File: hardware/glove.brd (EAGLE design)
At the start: 50.8 x 36.8 mm, 91 parts, among them J1 TC2030-JLINK-NL, J2 MICRO_USB_B_JST_MC5BR3-M404-4S, P1 DMP1045U, T0 WIREPAD1,6/0,8, T1 WIREPAD1,6/0,8, T2 WIREPAD1,6/0,8, T3 WIREPAD1,6/0,8, U1 NRF51822QF, U2 BNO055, U3 AT42QT1070, U4 MCP73831, U5 LP3855EMP-ADJ, X1 ABS05-32.768KHZ-9-T

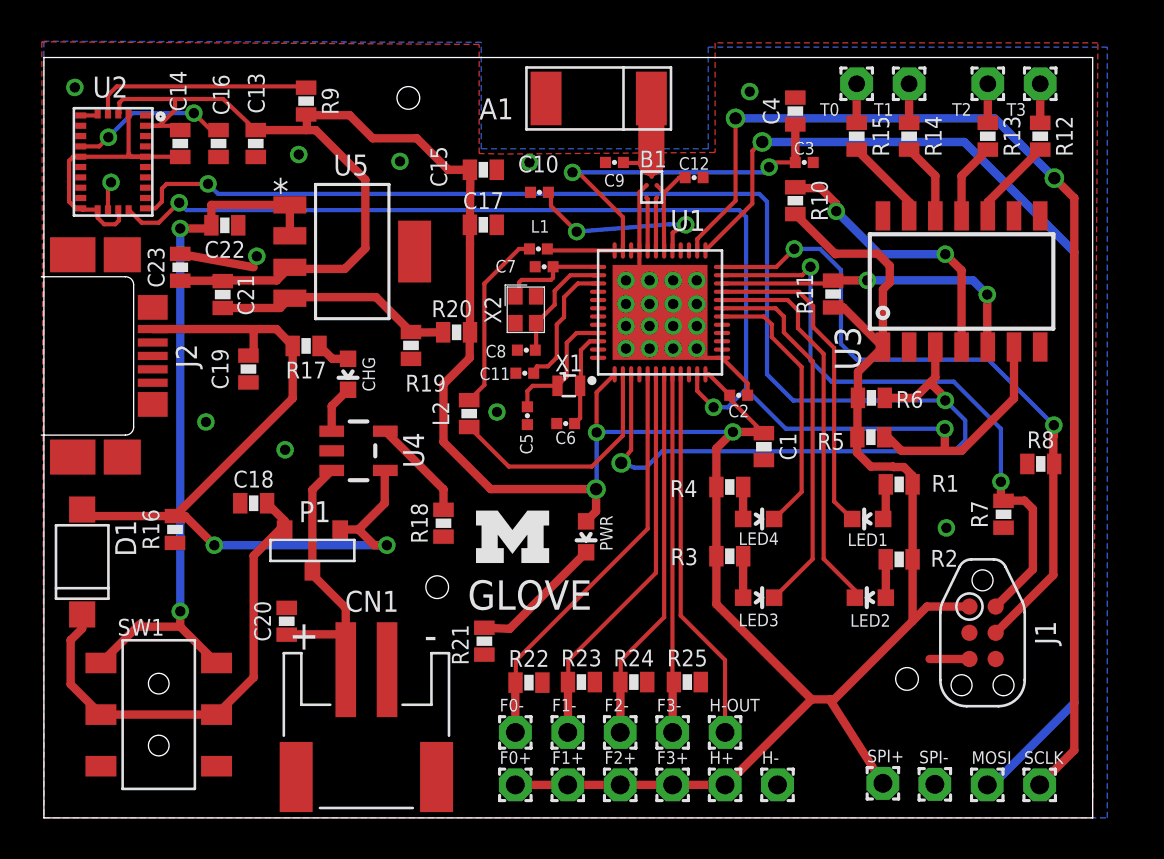
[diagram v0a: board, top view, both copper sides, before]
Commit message: turns out they're not quite done...damn
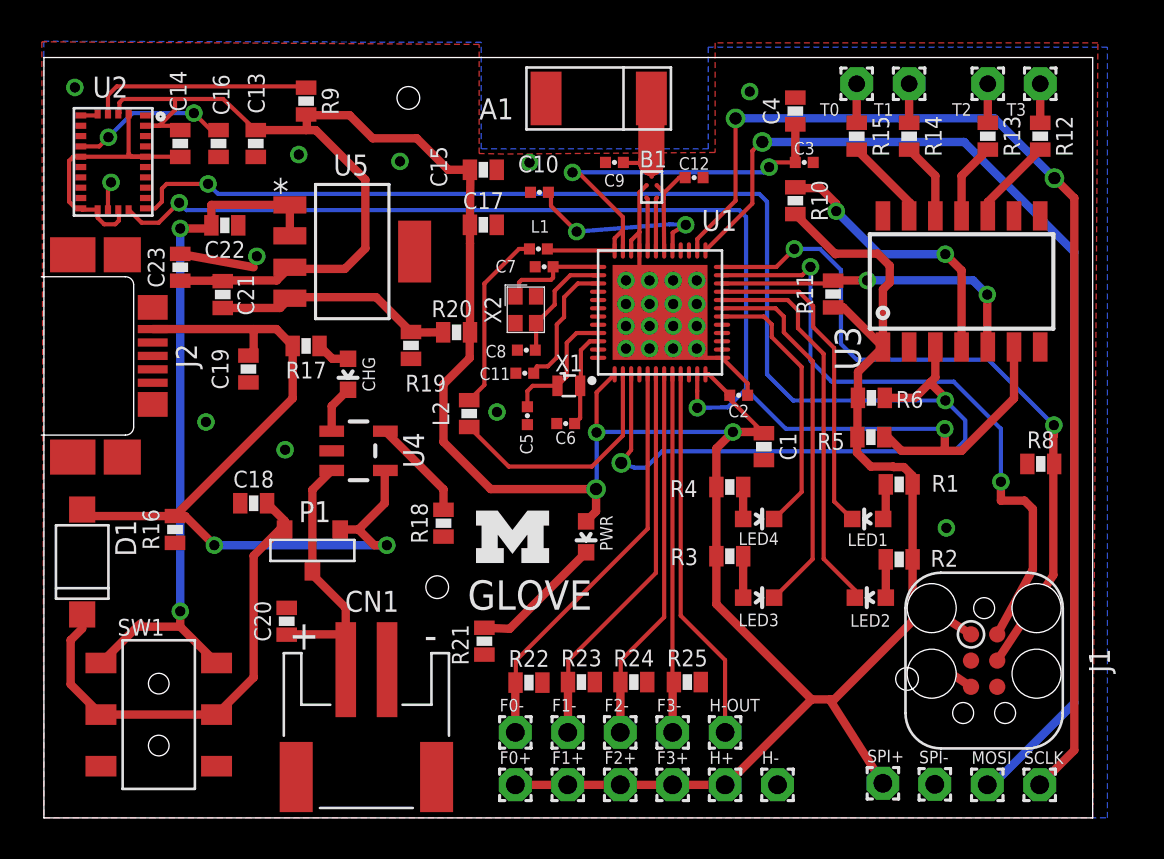
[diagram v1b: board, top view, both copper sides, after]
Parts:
- removed R7: 150, passives:0603-RES
- J1: value TC2030-JLINK-NL -> TC2030-JLINK-L; device connector:TC2030-IDC-NL -> connector:TC2030-IDC
- moved J1 1.35 mm to (45.5, 2.54)
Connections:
- net GND: no longer R7.1
- net N$19: no longer R7.2
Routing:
- net GND: track 33.6 -> 34.7 mm
- net N$19: track 30.2 -> 31.3 mm
- net N$30: track 33.4 -> 34.4 mm
- net N$16: track 21.5 -> 22.3 mm
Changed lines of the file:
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@@
 <?xml version="1.0" encoding="utf-8"?>
 <!DOCTYPE eagle SYSTEM "eagle.dtd">
-<eagle version="6.6.0">
+<eagle version="7.6.0">
 <drawing>
 <settings>
@@
 <pass name="Default">
 <param name="RoutingGrid" value="50mil"/>
+<param name="AutoGrid" value="1"/>
+<param name="Efforts" value="0"/>
+<param name="TopRouterVariant" value="1"/>
 <param name="tpViaShape" value="round"/>
 <param name="PrefDir.1" value="|"/>
@@
 <attribute name="VALUE" x="18.161" y="6.0198" size="1.27" layer="27" font="vector" rot="R180"/>
 </element>
-<element name="J1" library="connector" package="TC2030-IDC-NL" value="TC2030-JLINK-NL" x="45.466" y="3.8862" rot="R270"/>
+<element name="J1" library="connector" package="TC2030-IDC" value="TC2030-JLINK-L" x="45.5422" y="2.54" rot="R270"/>
 <element name="J2" library="connector" package="USB_MICRO_B-JST-MC5BR3-M404-4S-TB" value="MICRO_USB_B_JST_MC5BR3-M404-4S" x="1.397" y="17.2974" rot="R270">
 <attribute name="MOUSER" value="53X3655" x="1.397" y="17.2974" size="1.778" layer="27" rot="R270" display="off"/>
@@
 <attribute name="NAME" x="31.0134" y="7.9756" size="0.8128" layer="25" font="vector" ratio="12" rot="R180" align="bottom-center"/>
 </element>
-<element name="R7" library="passives" package="0603-RES" value="150" x="46.482" y="9.6266" smashed="yes" rot="R90">
-<attribute name="NAME" x="45.72" y="9.6266" size="0.8128" layer="25" font="vector" ratio="12" rot="R90" align="bottom-center"/>
-</element>
 <element name="R22" library="passives" package="0603-RES" value="20k" x="23.495" y="1.4732" smashed="yes">
 <attribute name="NAME" x="23.495" y="2.2352" size="0.8128" layer="25" font="vector" ratio="12" align="bottom-center"/>
@@
 <attribute name="MOUSER" value="949-NRF51822-QFAB-R7" x="29.845" y="19.4056" size="1.778" layer="27" rot="R90" display="off"/>
 <attribute name="DIGIKEY" value="1490-1032-1-ND" x="29.845" y="19.4056" size="1.778" layer="27" rot="R90" display="off"/>
-<attribute name="NAME" x="31.1912" y="24.3686" size="1.016" layer="25" font="vector" ratio="12" rot="R180" align="bottom-center"/>
+<attribute name="NAME" x="32.7152" y="24.3686" size="1.016" layer="25" font="vector" ratio="12" rot="R180" align="bottom-center"/>
 </element>
 <element name="U2" library="BNO055" package="LGA28R50P4X10_380X520X100" value="BNO055" x="3.3528" y="26.6954" smashed="yes" rot="R270">
@@
 <contactref element="C8" pad="2"/>
 <contactref element="R8" pad="1"/>
-<contactref element="R7" pad="1"/>
 <contactref element="J1" pad="5"/>
 <contactref element="U2" pad="6"/>
@@
 <vertex x="0" y="32.5374"/>
 </polygon>
-<wire x1="28.445" y1="22.4056" x2="28.845" y2="22.4056" width="0.2032" layer="1"/>
-<wire x1="28.845" y1="22.4056" x2="28.845" y2="25.2156" width="0.2032" layer="1"/>
+<wire x1="28.845" y1="22.4056" x2="28.845" y2="23.2918" width="0.2032" layer="1"/>
+<wire x1="28.845" y1="23.2918" x2="28.845" y2="25.2156" width="0.2032" layer="1"/>
 <wire x1="28.845" y1="25.2156" x2="29.1886" y2="25.5592" width="0.2032" layer="1"/>
 <wire x1="28.845" y1="22.4056" x2="28.845" y2="20.4056" width="0.2032" layer="1"/>
@@
 <via x="34.1884" y="30.099" extent="1-16" drill="0.5"/>
 <via x="43.7134" y="8.9662" extent="1-16" drill="0.5"/>
-<wire x1="42.9006" y1="2.6162" x2="44.831" y2="2.6162" width="0.4064" layer="1"/>
+<wire x1="42.9006" y1="2.6162" x2="44.9072" y2="1.27" width="0.4064" layer="1"/>
 <via x="28.194" y="20.955" extent="1-16" drill="0.5"/>
 <via x="29.337" y="20.955" extent="1-16" drill="0.5"/>
@@
 <wire x1="6.593" y1="26.9454" x2="6.604" y2="26.9344" width="0.2032" layer="1"/>
 <contactref element="R21" pad="1"/>
+<wire x1="28.445" y1="22.4056" x2="28.445" y2="22.8918" width="0.2032" layer="1"/>
+<wire x1="28.445" y1="22.8918" x2="28.845" y2="23.2918" width="0.2032" layer="1"/>
+<wire x1="43.1546" y1="-3.4544" x2="44.9072" y2="1.27" width="0" layer="19" extent="1-1"/>
 </signal>
 <signal name="N$14">
@@
 <contactref element="U1" pad="36"/>
 <contactref element="C3" pad="1"/>
-<wire x1="28.045" y1="22.4056" x2="27.645" y2="22.4056" width="0.2032" layer="1"/>
 <wire x1="36.3982" y1="28.5092" x2="36.39693125" y2="28.50793125" width="0.6096" layer="1"/>
 <via x="35.1282" y="26.4414" extent="1-16" drill="0.5"/>
 <via x="25.6032" y="26.1874" extent="1-16" drill="0.5"/>
-<wire x1="28.045" y1="24.025" x2="28.045" y2="22.4056" width="0.2032" layer="1"/>
+<wire x1="28.045" y1="24.025" x2="28.045" y2="23.3934" width="0.2032" layer="1"/>
+<wire x1="28.045" y1="23.3934" x2="28.045" y2="22.4056" width="0.2032" layer="1"/>
 <wire x1="35.1282" y1="26.4414" x2="34.8742" y2="26.1874" width="0.2032" layer="16"/>
 <wire x1="34.8742" y1="26.1874" x2="25.6032" y2="26.1874" width="0.2032" layer="16"/>
@@
 <wire x1="24.38526875" y1="22.479" x2="24.38526875" y2="22.4056" width="0.2032" layer="1"/>
 <wire x1="24.38526875" y1="22.4056" x2="27.645" y2="22.4056" width="0.2032" layer="1"/>
+<wire x1="27.645" y1="22.4056" x2="27.645" y2="22.9934" width="0.2032" layer="1"/>
+<wire x1="27.645" y1="22.9934" x2="28.045" y2="23.3934" width="0.2032" layer="1"/>
 </signal>
 <signal name="N$21">
@@
 <wire x1="12.7358" y1="28.2702" x2="12.7" y2="28.2344" width="0.2032" layer="1"/>
 <wire x1="42.0774" y1="4.4554" x2="42.0774" y2="7.4422" width="0.4064" layer="1"/>
-<wire x1="44.831" y1="5.1562" x2="42.7782" y2="5.1562" width="0.4064" layer="1"/>
+<wire x1="44.9072" y1="3.81" x2="42.7782" y2="5.1562" width="0.4064" layer="1"/>
 <wire x1="42.7782" y1="5.1562" x2="42.0774" y2="4.4554" width="0.4064" layer="1"/>
 <wire x1="42.0774" y1="7.4422" x2="42.0774" y2="11.0744" width="0.4064" layer="1"/>
@@
 <signal name="N$19">
 <contactref element="U1" pad="23"/>
-<contactref element="R7" pad="2"/>
 <contactref element="J1" pad="2"/>
 <via x="37.1314" y="21.612" extent="1-16" drill="0.5"/>
 <wire x1="38.1508" y1="16.0528" x2="44.069" y2="16.0528" width="0.2032" layer="16"/>
 <via x="46.355" y="11.2014" extent="1-16" drill="0.5"/>
-<wire x1="47.9044" y1="6.9596" x2="46.101" y2="5.1562" width="0.4064" layer="1"/>
+<wire x1="47.9044" y1="6.9596" x2="46.1772" y2="3.81" width="0.4064" layer="1"/>
 <wire x1="47.9044" y1="6.9596" x2="47.9044" y2="9.8806" width="0.4064" layer="1"/>
 <wire x1="47.9044" y1="9.8806" x2="47.498" y2="10.287" width="0.4064" layer="1"/>
-<wire x1="46.4462" y1="10.3124" x2="46.482" y2="10.2766" width="0.4064" layer="1"/>
-<wire x1="47.498" y1="10.287" x2="46.4924" y2="10.287" width="0.4064" layer="1"/>
-<wire x1="46.4924" y1="10.287" x2="46.482" y2="10.2766" width="0.4064" layer="1"/>
+<wire x1="47.498" y1="10.287" x2="46.355" y2="10.287" width="0.4064" layer="1"/>
 <wire x1="32.845" y1="21.2056" x2="36.725" y2="21.2056" width="0.2032" layer="1"/>
 <wire x1="36.725" y1="21.2056" x2="37.1314" y2="21.612" width="0.2032" layer="1"/>
 <wire x1="37.1314" y1="21.612" x2="37.1314" y2="17.0722" width="0.2032" layer="16"/>
 <wire x1="37.1314" y1="17.0722" x2="38.1508" y2="16.0528" width="0.2032" layer="16"/>
-<wire x1="46.355" y1="11.2014" x2="46.355" y2="10.4036" width="0.4064" layer="1"/>
-<wire x1="46.355" y1="10.4036" x2="46.482" y2="10.2766" width="0.4064" layer="1"/>
 <wire x1="46.355" y1="11.2014" x2="46.355" y2="13.7668" width="0.2032" layer="16"/>
 <wire x1="46.355" y1="13.7668" x2="44.069" y2="16.0528" width="0.2032" layer="16"/>
+<wire x1="46.355" y1="10.287" x2="46.355" y2="11.2014" width="0.4064" layer="1"/>
 </signal>
 <signal name="N$30">
@@
 <wire x1="32.845" y1="21.6056" x2="35.474" y2="21.6056" width="0.2032" layer="1"/>
 <wire x1="35.474" y1="21.6056" x2="36.3474" y2="22.479" width="0.2032" layer="1"/>
-<wire x1="48.895" y1="6.6802" x2="46.101" y2="3.8862" width="0.4064" layer="1"/>
+<wire x1="48.895" y1="6.6802" x2="46.1772" y2="2.54" width="0.4064" layer="1"/>
 <wire x1="48.895" y1="12.0246" x2="48.9354" y2="12.065" width="0.4064" layer="1"/>
 <wire x1="48.895" y1="12.0246" x2="48.895" y2="13.4366" width="0.4064" layer="1"/>
@@
 <wire x1="6.5532" y1="24.7142" x2="6.9088" y2="24.3586" width="0.2032" layer="16"/>
 <wire x1="6.9088" y1="24.3586" x2="33.6804" y2="24.3586" width="0.2032" layer="16"/>
-<via x="32.4358" y="14.8082" extent="1-16" drill="0.5"/>
+<via x="31.6484" y="14.7828" extent="1-16" drill="0.5"/>
 <wire x1="33.6804" y1="24.3586" x2="34.0106" y2="24.0284" width="0.2032" layer="16"/>
 <wire x1="34.0106" y1="24.0284" x2="34.0106" y2="15.6972" width="0.2032" layer="16"/>
@@
 <via x="43.6372" y="13.7668" extent="1-16" drill="0.5"/>
 <wire x1="43.6372" y1="13.7668" x2="43.6372" y2="12.7" width="0.4064" layer="1"/>
-<wire x1="32.4358" y1="14.8082" x2="33.1216" y2="14.8082" width="0.2032" layer="16"/>
+<wire x1="31.6484" y1="14.7828" x2="33.1216" y2="14.8082" width="0.2032" layer="16"/>
 <wire x1="33.1216" y1="14.8082" x2="34.0106" y2="15.6972" width="0.2032" layer="16"/>
 <wire x1="31.645" y1="16.4056" x2="31.645" y2="15.599" width="0.2032" layer="1"/>
-<wire x1="31.645" y1="15.599" x2="32.4358" y2="14.8082" width="0.2032" layer="1"/>
+<wire x1="31.645" y1="15.599" x2="31.6484" y2="14.7828" width="0.2032" layer="1"/>
 <wire x1="40.7058" y1="13.3604" x2="40.6804" y2="13.5636" width="0.4064" layer="1"/>
 <wire x1="40.6804" y1="13.5636" x2="41.544" y2="12.7" width="0.4064" layer="1"/>
